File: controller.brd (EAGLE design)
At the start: 100 x 80 mm, 8 parts, among them X1 PUSHBUTTON_LED

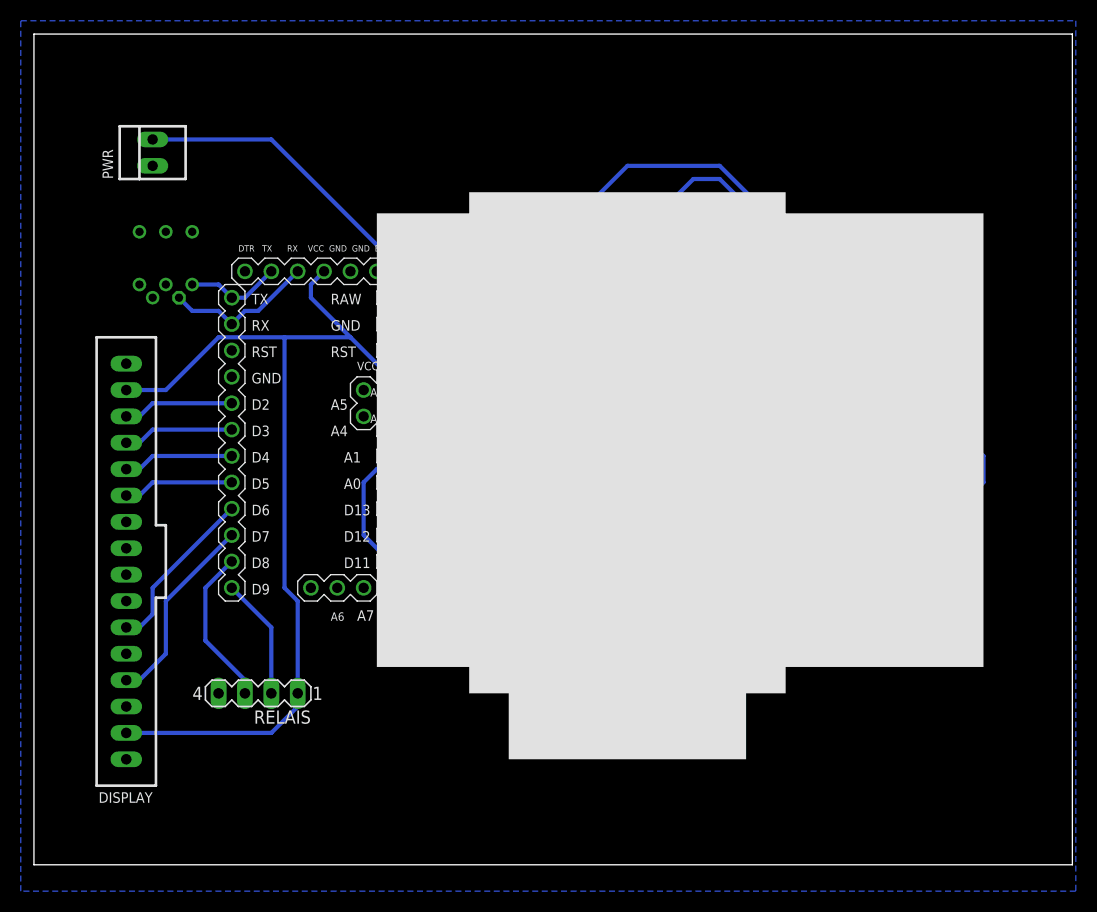
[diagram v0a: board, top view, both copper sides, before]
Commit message: board layout, should work
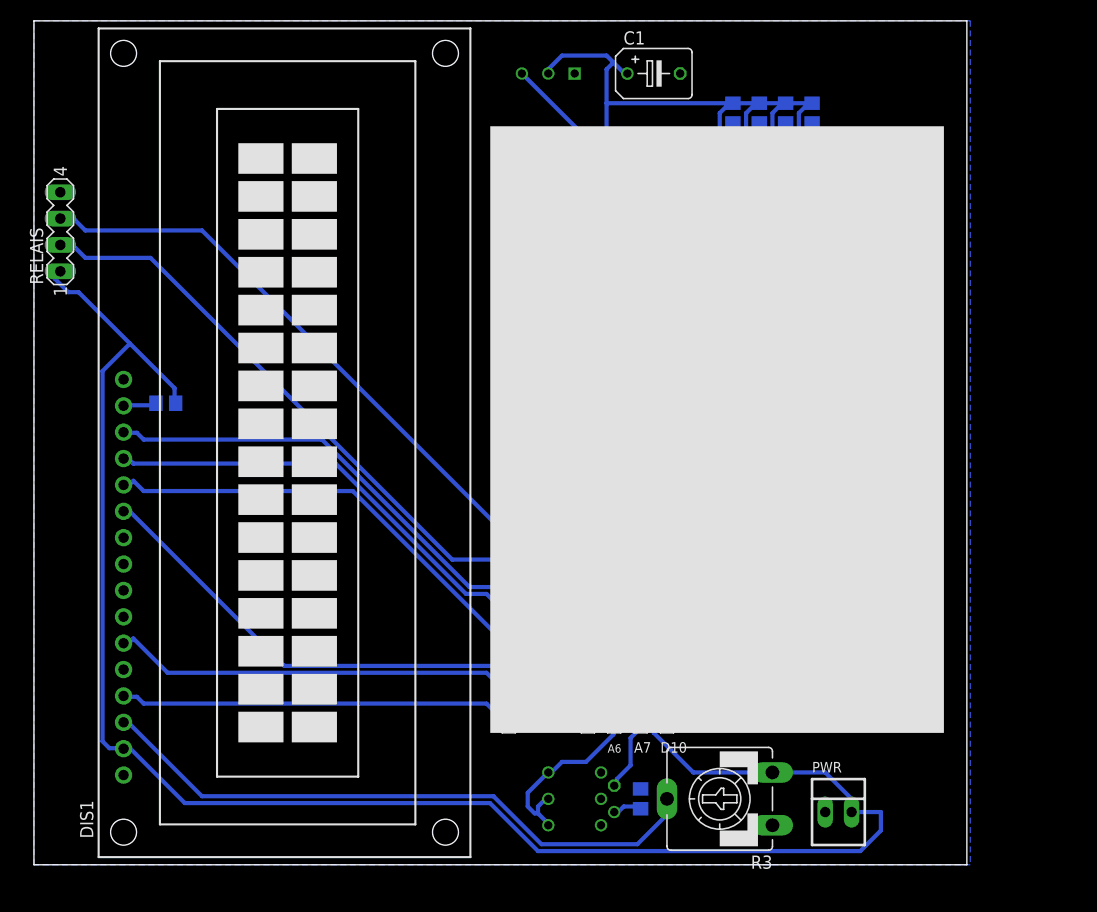
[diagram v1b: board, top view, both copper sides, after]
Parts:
- removed DISPLAY: C-GRID-16-70543, con-molex:70543-16
- removed U$2: LEVELSHIFTER, local:2*6DIP
- added C1: 47u, rcl:B45181B
- added DIS1: TUXGR_16X2_R2, display-lcd:TUXGR_16X2_R2
- added Q1, Q2, Q3, Q4: BSS138, local:SOT23
- added R1, R2: 220, eagle-ltspice:R0805
- added R10, R11, R4, R5, R6, R7, R8, R9: 10k, eagle-ltspice:R0805
- added R3: 10k, pot:CA9V
- added U$4: PWR_CONV, local:PWR_CONV
- moved PWR 91.6 mm to (77.5, 5.08), turned to 0 degrees
- moved X1 65.3 mm to (52.1, 6.35), turned to 180 degrees
- moved U$3 52.2 mm to (87.6, 71.1), turned to 180 degrees
- moved RELAIS 48.4 mm to (2.54, 61.0), turned to 90 degrees
- moved U$1 36.1 mm to (68.6, 27.9), flipped to the bottom, turned to 180 degrees
- moved ARDUINO1 29.5 mm to (49.5, 33.0)
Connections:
- removed net N$6: U$2.P$7, U$3.SDA
- removed net N$9: ARDUINO1.D8, RELAIS.3
- new net N$17: ARDUINO1.A6, X1.P$2, X1.P$4, X1.P$6
- new net N$18: DIS1.15, R1.1
- new net N$19: ARDUINO1.D4, DIS1.14
- new net SS_RFID_3V3: Q2.2, R6.1, U$3.SDA
- net +3V3: now also C1.+, Q1.1, Q2.1, Q3.1, Q4.1, R10.2, R4.2, R6.2, R8.2, U$4.VOUT; no longer U$2.P$12
- net +5V: now also DIS1.2, PWR.2, R1.2, R11.2, R3.E, R5.2, R7.2, R9.2, U$4.VIN; no longer DISPLAY.15, DISPLAY.2, U$2.P$6
- net GND: now also C1.-, DIS1.1, DIS1.16, DIS1.5, R2.2, R3.A, U$4.GND, X1.P$5; no longer DISPLAY.1, DISPLAY.16, DISPLAY.5, U$2.P$11, U$2.P$5, X1.P$2, X1.P$4, X1.P$6, X1.P$C
- net MISO: now also Q4.3, R11.1; no longer U$2.P$3
- net MOSI: now also Q3.3, R9.1; no longer U$2.P$2
- net N$1: now also R2.1, X1.P$C; no longer ARDUINO1.RX, ARDUINO1.RX@1, X1.P$A
- net N$10: now also ARDUINO1.D7, DIS1.11; no longer ARDUINO1.D5, DISPLAY.11
- net N$11: now also ARDUINO1.A7, X1.P$A; no longer ARDUINO1.TX, ARDUINO1.TX@1, X1.P$5
- net N$12: now also ARDUINO1.D8, DIS1.6; no longer ARDUINO1.D6, DISPLAY.6
- net N$13: now also ARDUINO1.D9, DIS1.4; no longer ARDUINO1.D7, DISPLAY.4
- net N$14: now also ARDUINO1.D6, DIS1.12; no longer ARDUINO1.D4, DISPLAY.12
- net N$15: now also RELAIS.2; no longer DISPLAY.13
- net N$16: now also RELAIS.3; no longer DISPLAY.14
- net N$2: now also Q1.2, R4.1; no longer U$2.P$10
- net N$3: now also Q3.2, R8.1; no longer U$2.P$8
- net N$4: now also Q4.2, R10.1; no longer U$2.P$9
- net N$5: now also ARDUINO1.A0; no longer ARDUINO1.A3
- net N$7: now also ARDUINO1.D5, DIS1.13; no longer ARDUINO1.RAW, PWR.2
- net N$8: now also DIS1.3, R3.S; no longer ARDUINO1.D9, RELAIS.2
- net SCK: now also Q1.3, R5.1; no longer U$2.P$4
- net SS_RFID: now also Q2.3, R7.1; no longer U$2.P$1
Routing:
- net +5V: track 156.1 -> 285.0 mm, vias 0 -> 2
- net +3V3: track 5.61 -> 79.8 mm
- net N$8: track 11.7 -> 59.9 mm
- net N$15: track 10.7 -> 55.9 mm
- net N$16: track 10.7 -> 55.9 mm
- net N$19: track 0.00 -> 43.3 mm
- net N$14: track 10.7 -> 43.9 mm
- net N$10: track 10.7 -> 43.5 mm
- net MOSI: track 92.0 -> 61.8 mm
- net N$5: track 32.0 -> 8.45 mm
- net SCK: track 73.5 -> 50.1 mm
- net N$12: track 16.4 -> 39.6 mm
- net N$13: track 18.9 -> 38.0 mm
- net SS_RFID: track 45.2 -> 64.0 mm
- net N$17: track 0.00 -> 18.8 mm
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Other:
- board size 100 x 80 mm -> 89.8 x 81.3 mm
